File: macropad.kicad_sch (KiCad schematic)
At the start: 7 parts, among them SW1 SW_Push, SW2 SW_Push, SW3 SW_Push, SW4 SW_Push, U1 XIAO-RP2040-DIP

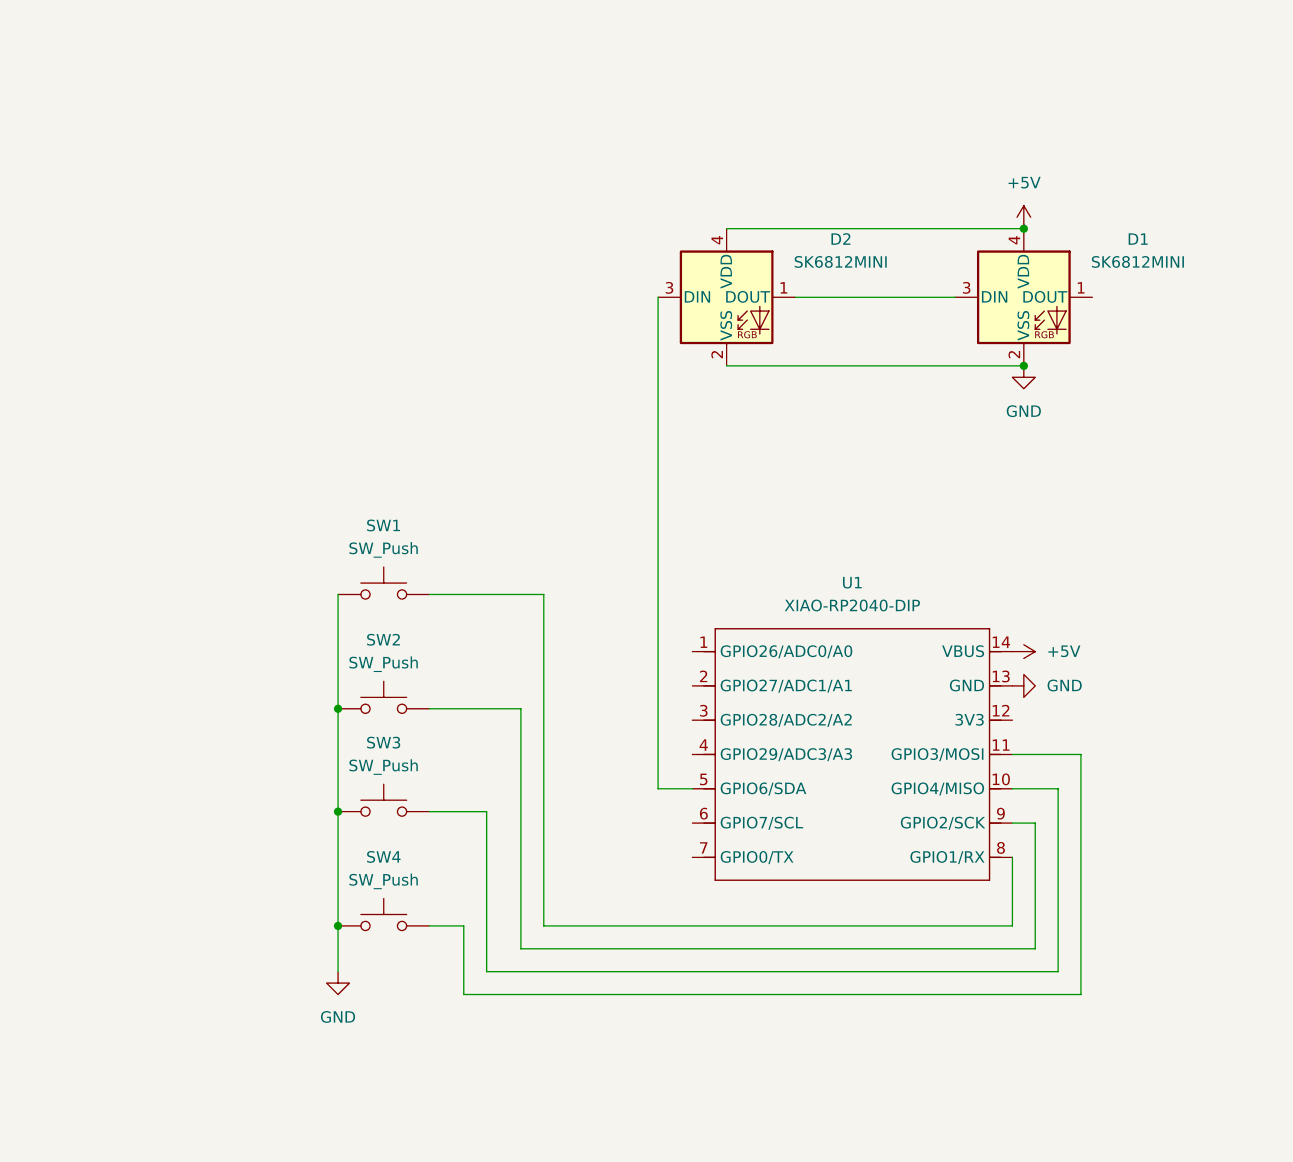
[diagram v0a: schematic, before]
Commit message: UPDATE:added pcb case and other stuffz!!!
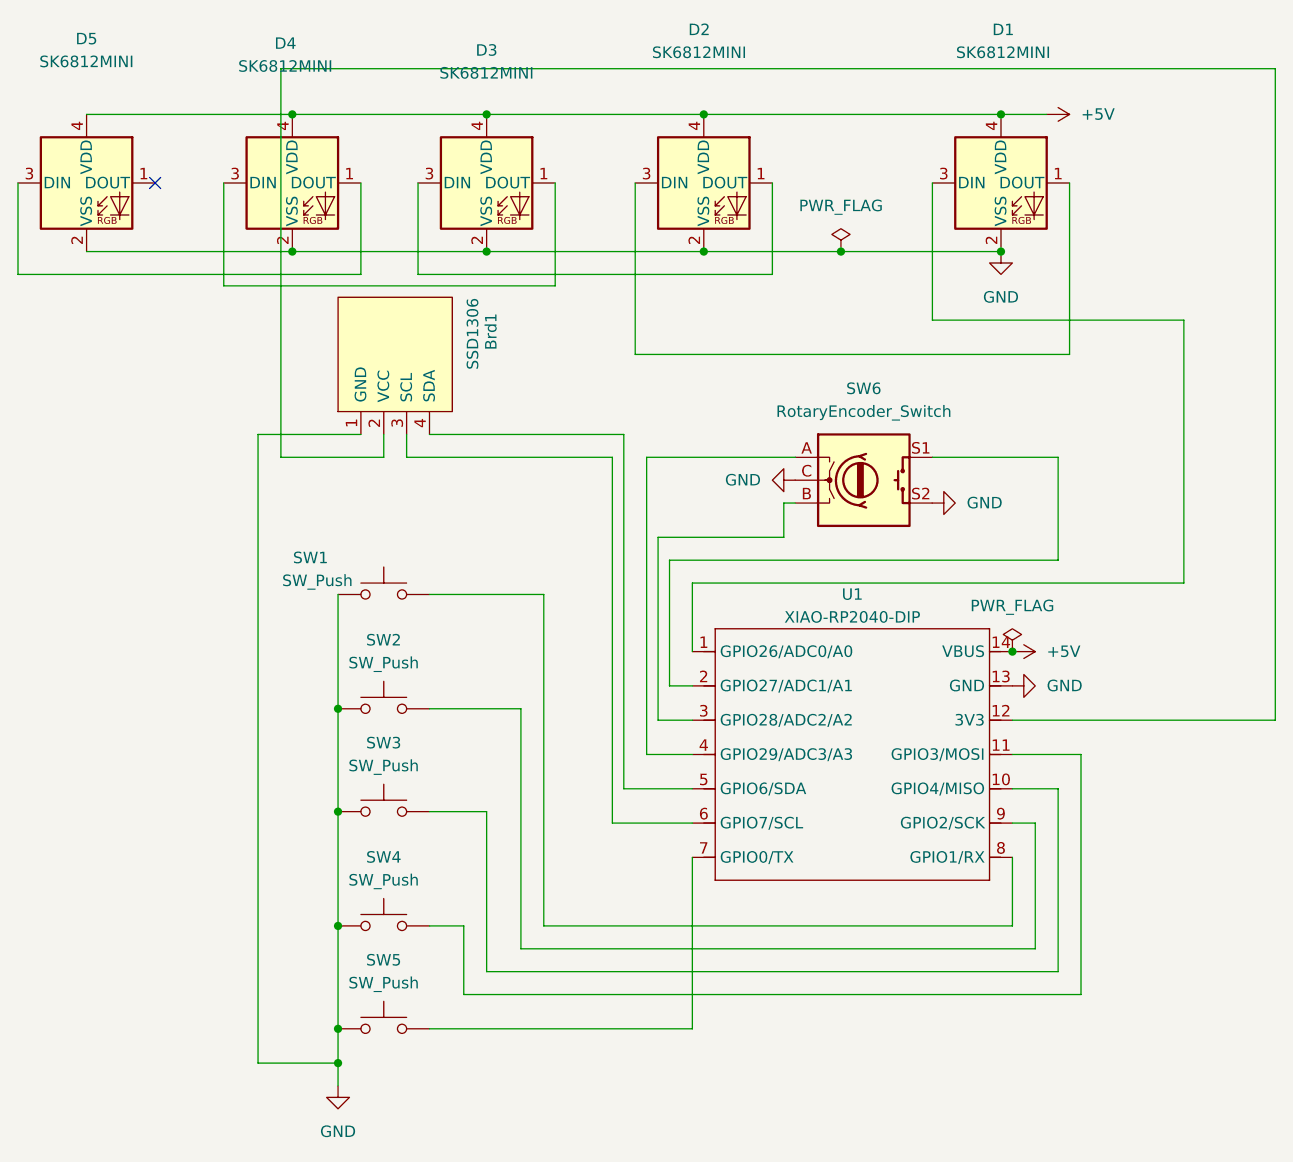
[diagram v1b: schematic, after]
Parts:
- added Brd1: SSD1306, OLED:SSD1306-0.91-OLED-4pin-128x32, symbol OLED:SSD1306
- added D3, D4, D5: SK6812MINI, LED_SMD:LED_SK6812MINI_PLCC4_3.5x3.5mm_P1.75mm, symbol LED:SK6812MINI
- added SW5: SW_Push, Button_Switch_Keyboard:SW_Cherry_MX_1.00u_PCB, symbol Switch:SW_Push
- added SW6: RotaryEncoder_Switch, Rotary_Encoder:RotaryEncoder_Alps_EC11E-Switch_Vertical_H20mm, symbol Device:RotaryEncoder_Switch
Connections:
- net +5V: now also D3.4 (VDD), D4.4 (VDD), D5.4 (VDD)
- net GND: now also Brd1.1 (GND), D3.2 (VSS), D4.2 (VSS), D5.2 (VSS), SW5.1, SW6.C, SW6.S2
- net at D2.1 (DOUT): now also D3.3 (DIN); no longer D1.3 (DIN)
- net at D2.3 (DIN): now also D1.1 (DOUT); no longer U1.5 (GPIO6/SDA)
- net at U1.1 (GPIO26/ADC0/A0): now also D1.3 (DIN)
- net at U1.12 (3V3): now also Brd1.2 (VCC)
- net at U1.2 (GPIO27/ADC1/A1): now also SW6.S1
- net at U1.3 (GPIO28/ADC2/A2): now also SW6.B
- net at U1.4 (GPIO29/ADC3/A3): now also SW6.A
- net at U1.6 (GPIO7/SCL): now also Brd1.3 (SCL)
- net at U1.7 (GPIO0/TX): now also SW5.2
- new net: D4.1 (DOUT), D5.3 (DIN)
- new net: Brd1.4 (SDA), U1.5 (GPIO6/SDA)
- new net: D3.1 (DOUT), D4.3 (DIN)
- no-connect marks 0 -> 1
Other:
- moved on the sheet: D1, D2
